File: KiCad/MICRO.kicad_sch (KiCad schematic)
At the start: 6 parts, among them U7 PIC32MX250F128D-IPT

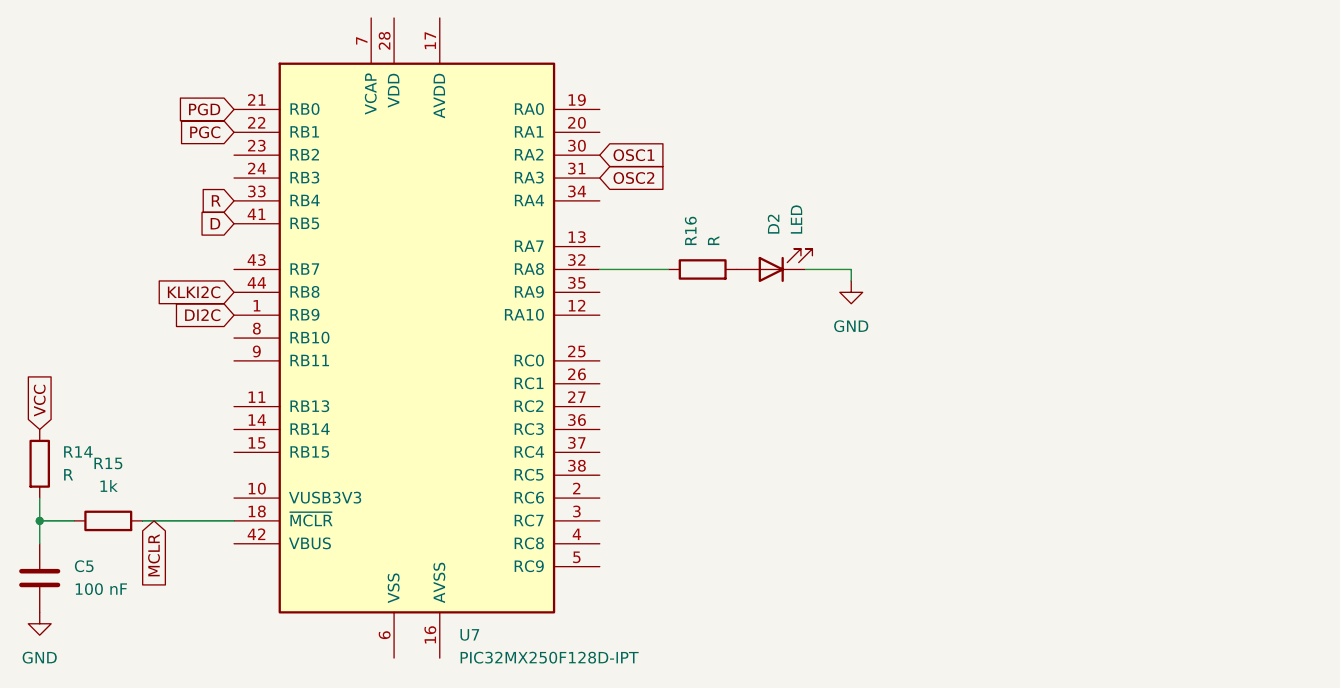
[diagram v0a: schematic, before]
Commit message: calefactor-Usart
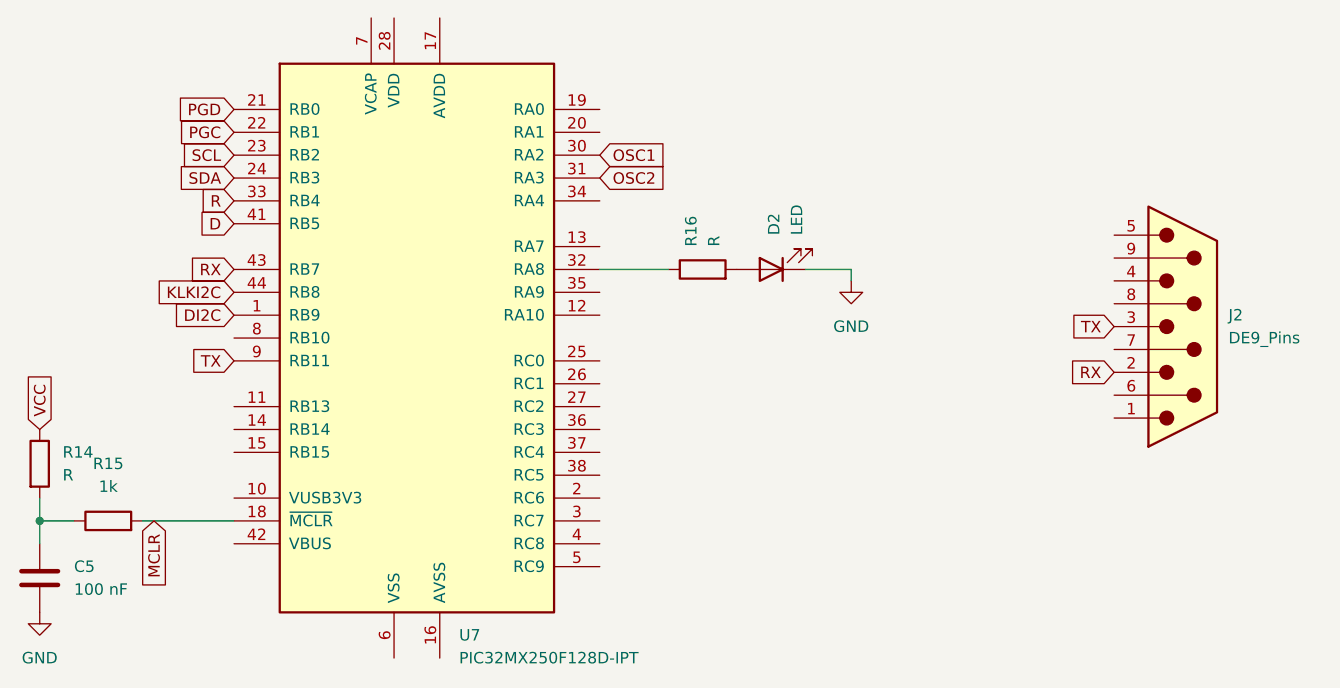
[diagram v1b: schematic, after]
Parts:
- added J2: DE9_Pins, symbol Connector:DE9_Pins
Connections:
- net SCL: now reaches U7.23 (RB2)
- net SDA: now reaches U7.24 (RB3)
- net RX: now reaches U7.43 (RB7)
- net RX: now also J2.2
- net TX: now reaches U7.9 (RB11)
- net TX: now also J2.3
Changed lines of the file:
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@@
+		)
+	)
+	(global_label "TX"
+		(shape input)
+		(at 123.19 92.71 180)
+		(fields_autoplaced yes)
+		(effects
+			(font
+				(size 1.27 1.27)
+			)
+			(justify right)
+		)
+		(property "Intersheetrefs" "${INTERSHEET_REFS}"
+			(at 118.0277 92.71 0)
+			(effects
+				(font
+					(size 1.27 1.27)
+				)
+				(justify right)
+				(hide yes)
+			)
+		)
+	)
+	(global_label "SDA"
+		(shape input)
+		(at 123.19 72.39 180)
+		(fields_autoplaced yes)
+		(effects
+			(font
+				(size 1.27 1.27)
+			)
+			(justify right)
+		)
+		(property "Intersheetrefs" "${INTERSHEET_REFS}"
+			(at 116.6367 72.39 0)
+			(effects
+				(font
+					(size 1.27 1.27)
+				)
+				(justify right)
+				(hide yes)
+			)
 		)
 	)
@@
 		)
 	)
+	(global_label "TX"
+		(shape input)
+		(at 220.98 88.9 180)
+		(fields_autoplaced yes)
+		(effects
+			(font
+				(size 1.27 1.27)
+			)
+			(justify right)
+		)
+		(property "Intersheetrefs" "${INTERSHEET_REFS}"
+			(at 215.8177 88.9 0)
+			(effects
+				(font
+					(size 1.27 1.27)
+				)
+				(justify right)
+				(hide yes)
+			)
+		)
+	)
 	(global_label "D"
 		(shape input)
@@
 		)
 	)
+	(global_label "SCL"
+		(shape input)
+		(at 123.19 69.85 180)
+		(fields_autoplaced yes)
+		(effects
+			(font
+				(size 1.27 1.27)
+			)
+			(justify right)
+		)
+		(property "Intersheetrefs" "${INTERSHEET_REFS}"
+			(at 116.6972 69.85 0)
+			(effects
+				(font
+					(size 1.27 1.27)
+				)
+				(justify right)
+				(hide yes)
+			)
+		)
+	)
 	(global_label "OSC1"
 		(shape input)
@@
 		)
 	)
+	(global_label "RX"
+		(shape input)
+		(at 123.19 82.55 180)
+		(fields_autoplaced yes)
+		(effects
+			(font
+				(size 1.27 1.27)
+			)
+			(justify right)
+		)
+		(property "Intersheetrefs" "${INTERSHEET_REFS}"
+			(at 117.7253 82.55 0)
+			(effects
+				(font
+					(size 1.27 1.27)
+				)
+				(justify right)
+				(hide yes)
+			)
+		)
+	)
+	(global_label "RX"
+		(shape input)
+		(at 220.98 93.98 180)
+		(fields_autoplaced yes)
+		(effects
+			(font
+				(size 1.27 1.27)
+			)
+			(justify right)
+		)
+		(property "Intersheetrefs" "${INTERSHEET_REFS}"
+			(at 215.5153 93.98 0)
+			(effects
+				(font
+					(size 1.27 1.27)
+				)
+				(justify right)
+				(hide yes)
+			)
+		)
+	)
 	(global_label "MCLR"
 		(shape input)
@@
 			)
 		)
+	)
+	(symbol
+		(lib_id "Connector:DE9_Pins")
+		(at 228.6 88.9 0)
+		(unit 1)
+		(exclude_from_sim no)
+		(in_bom yes)
+		(on_board yes)
+		(dnp no)
+		(fields_autoplaced yes)
+		(property "Reference" "J2"
+			(at 233.68 87.6299 0)
+			(effects
+				(font
+					(size 1.27 1.27)
+				)
+				(justify left)
+			)
+		)
+		(property "Value" "DE9_Pins"
+			(at 233.68 90.1699 0)
+			(effects
+				(font
+					(size 1.27 1.27)
+				)
+				(justify left)
+			)
+		)
+		(property "Footprint" ""
+			(at 228.6 88.9 0)
+			(effects
+				(font
+					(size 1.27 1.27)
+				)
+				(hide yes)
+			)
+		)
+		(property "Datasheet" "~"
+			(at 228.6 88.9 0)
+			(effects
+				(font
+					(size 1.27 1.27)
+				)
+				(hide yes)
+			)
+		)
+		(property "Description" "9-pin D-SUB connector, pins (male)"
+			(at 228.6 88.9 0)
+			(effects
+				(font
+					(size 1.27 1.27)
+				)
+				(hide yes)
+			)
+		)
+		(pin "4"
+		)
+		(pin "7"
+		)
+		(pin "1"
+		)
+		(pin "3"
+		)
+		(pin "2"
+		)
+		(pin "9"
+		)
+		(pin "8"
+		)
+		(pin "5"
+		)
+		(pin "6"
+		)
+		(instances
+			(project ""
+				(path "/9b9f005f-0621-4675-bd4e-683e7082b120/2f39354d-8df5-4269-96cb-5875be0a8958"
+					(reference "J2")
+					(unit 1)
+				)
+			)
+		)
